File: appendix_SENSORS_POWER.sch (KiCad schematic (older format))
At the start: 58 parts, among them J401 Conn_01x02, J402 Conn_01x02, J403 Screw_Terminal_01x02, J404 Conn_01x02, J405 Conn_01x02, J406 Screw_Terminal_01x02, J407 Conn_01x02, J408 Conn_01x02, J409 Conn_01x02, J410 Conn_01x02, J411 Conn_01x02, J605 Conn_01x03, J606 Conn_01x03, T401 PMV40UN2, T402 BUK963R3-60E, T403 BUK963R3-60E, T404 PMV40UN2, T405 PMV40UN2

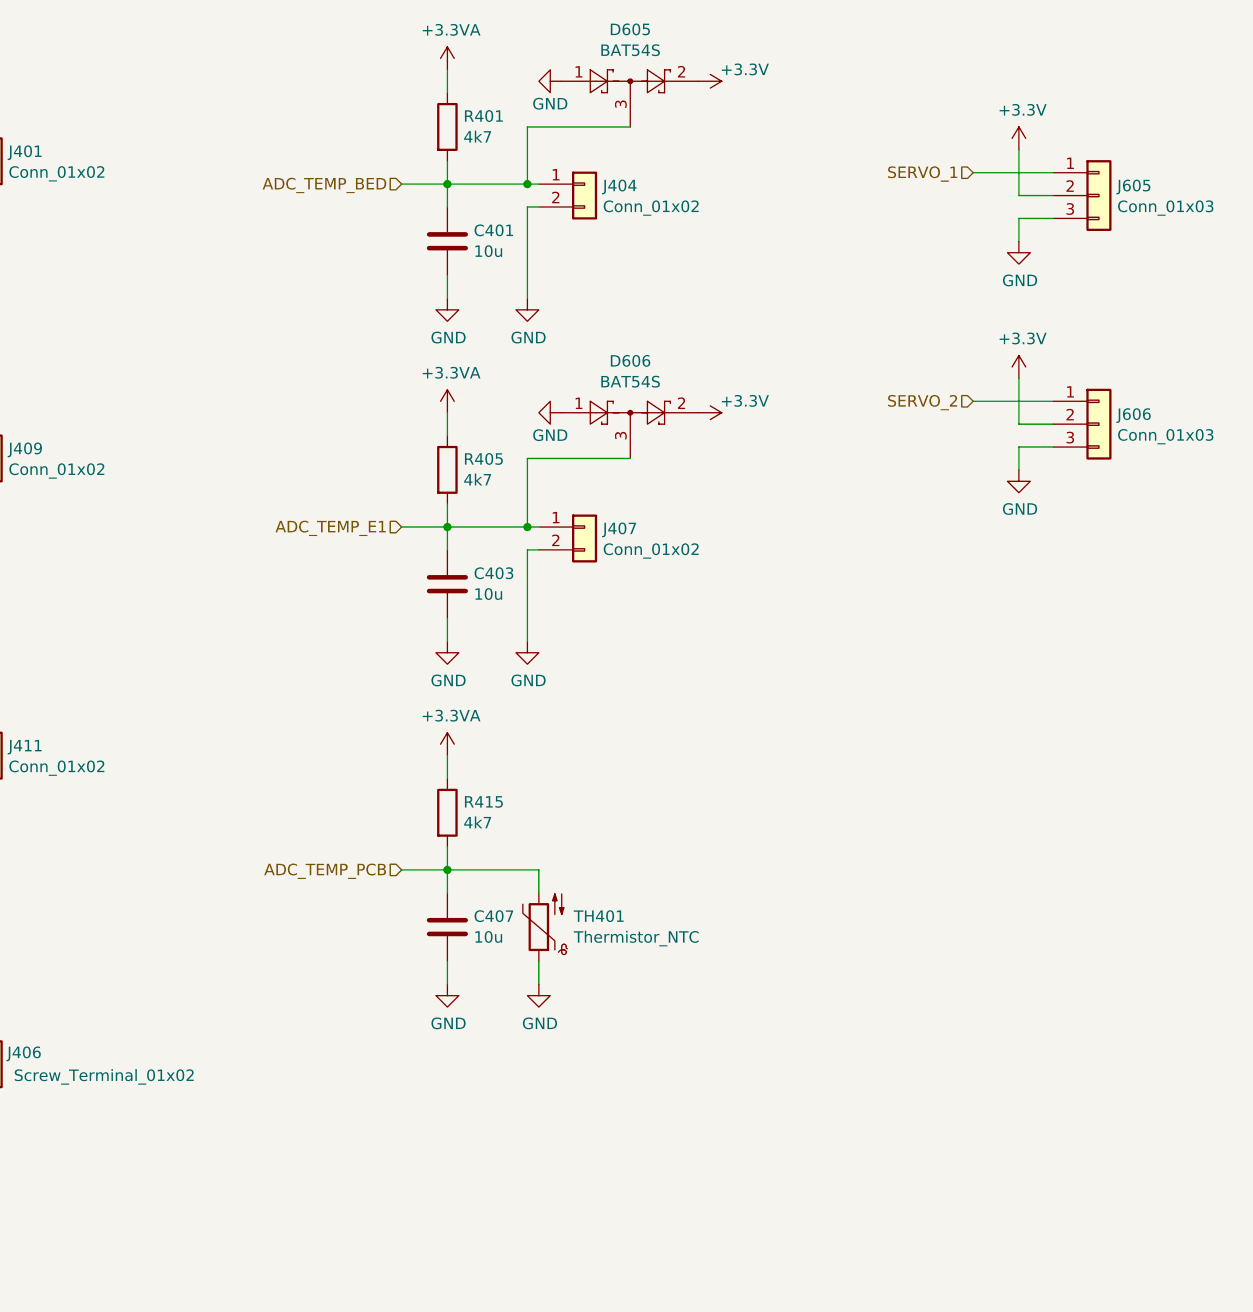
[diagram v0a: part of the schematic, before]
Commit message: finished up for final review
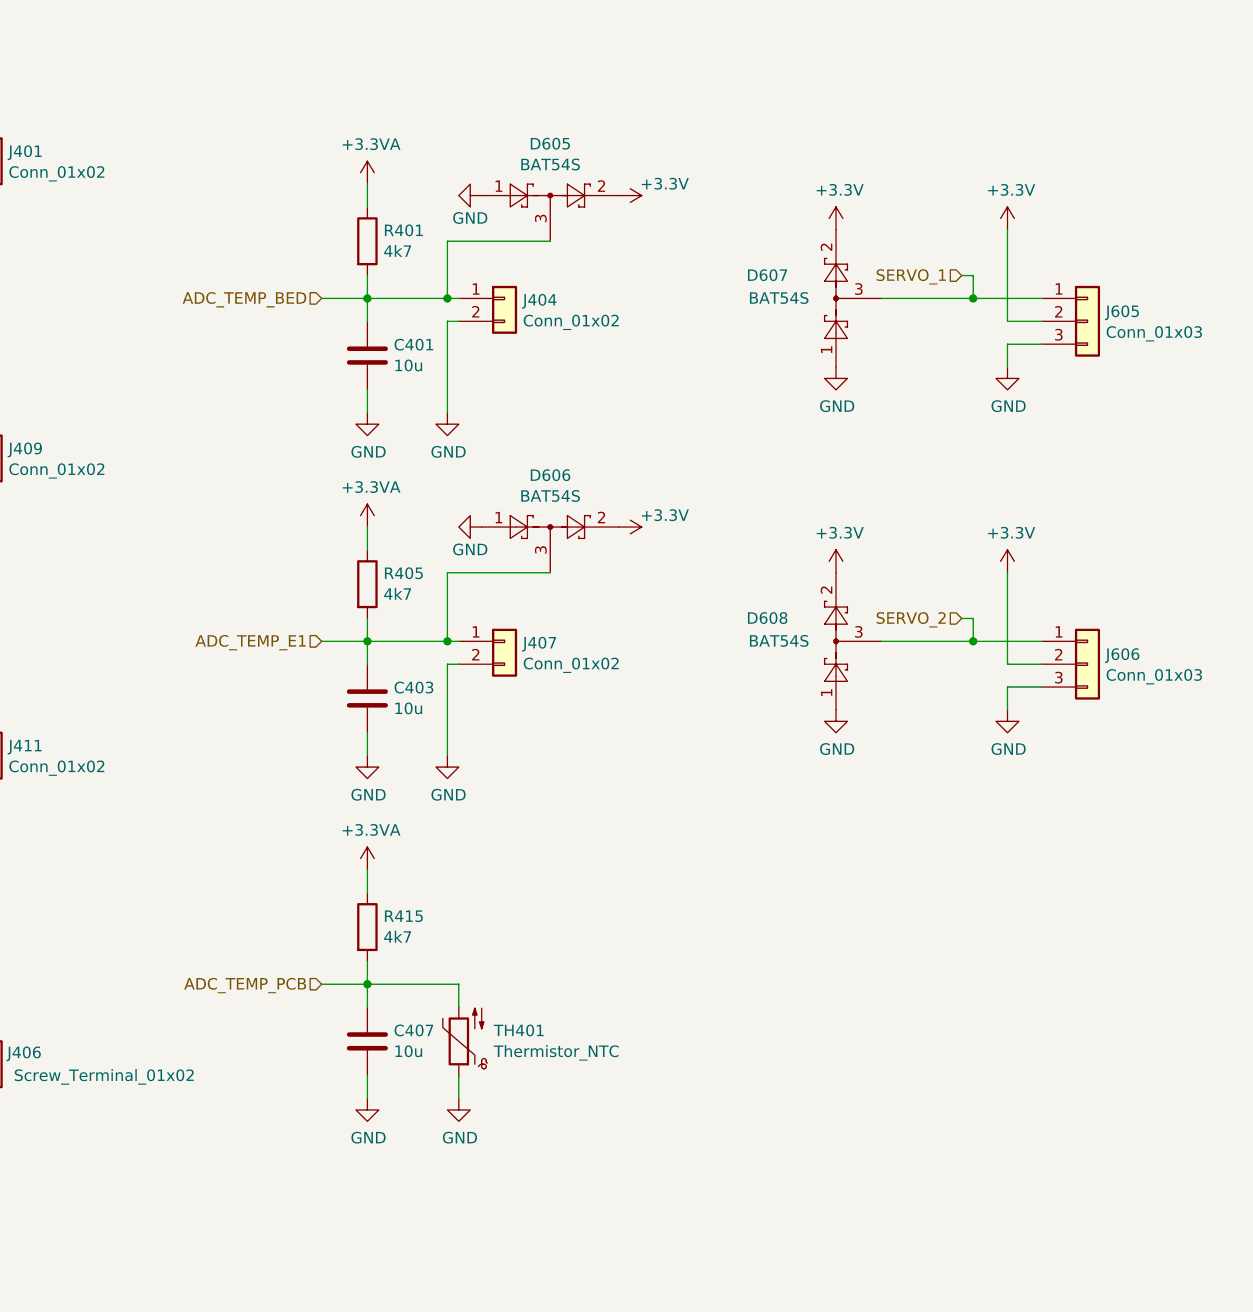
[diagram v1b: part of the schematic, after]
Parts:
- added D607, D608: BAT54S, Package_TO_SOT_SMD:SOT-23, symbol Diode:BAT54S
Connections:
- net +3V3: now also D607.2, D608.2
- net GND: now also D607.1, D608.1
- net SERVO_1: now also D607.3
- net SERVO_2: now also D608.3
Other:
- moved on the sheet: C401, C403, C407, D605, D606, J404, J407, J605, J606, R401, R405, R415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
